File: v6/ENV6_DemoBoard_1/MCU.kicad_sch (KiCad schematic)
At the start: 41 parts, among them J401 Pico Debugger (SWD), J402 Conn_01x04_Pin, U401 RP2354B, U402 Pi-Radio, U403 W25Q16JVUXIQ, Y401 KX7_QRZ

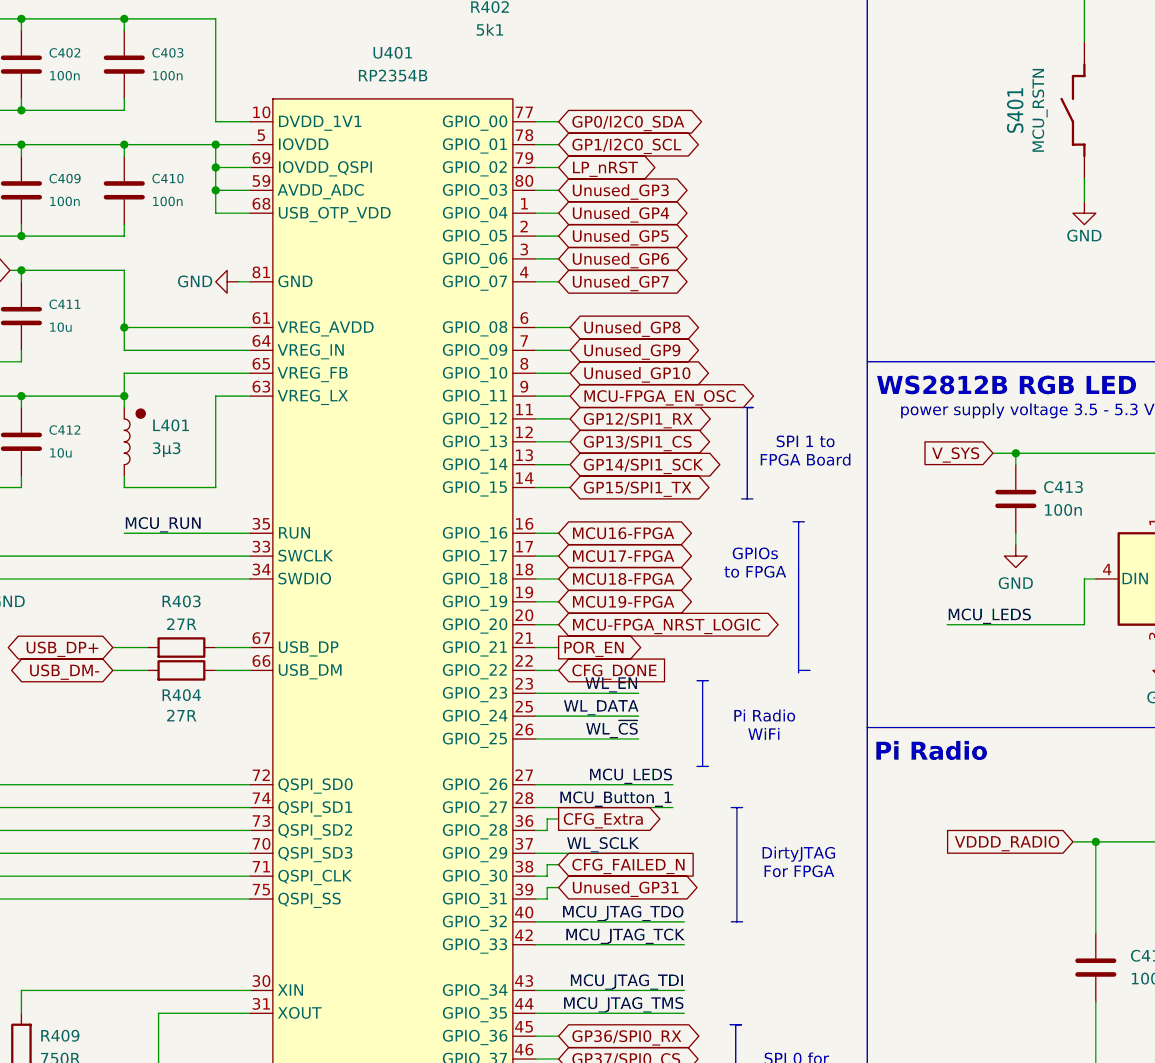
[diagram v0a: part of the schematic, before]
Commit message: first rev Base Board pcb layout
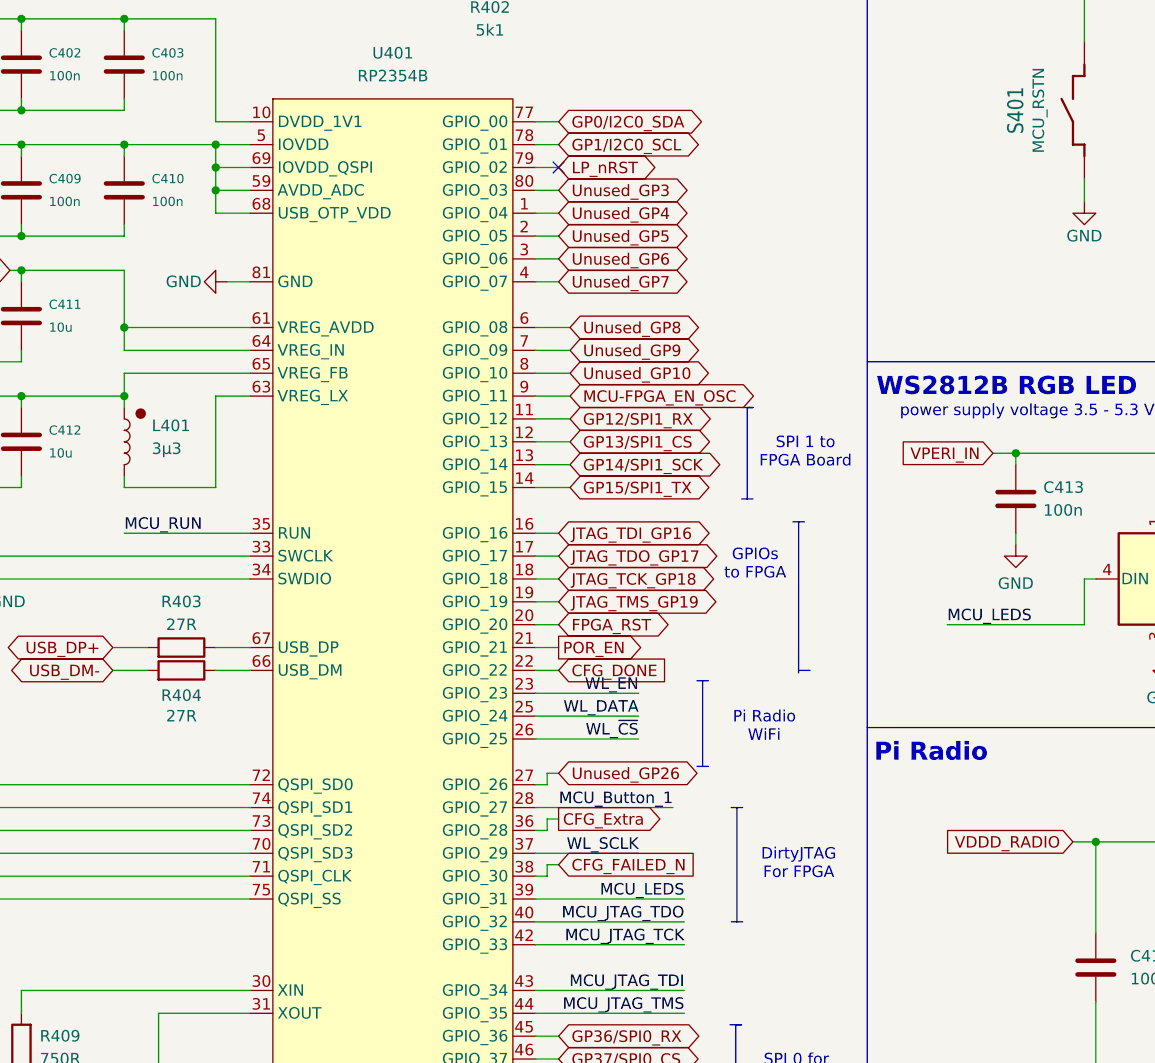
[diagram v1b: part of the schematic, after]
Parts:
- J401: footprint Connector_PinHeader_2.54mm:PinHeader_1x03_P2.54mm_Vertical -> Connector_PinHeader_2.00mm:PinHeader_1x03_P2.00mm_Vertical
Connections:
- net Unused_GP31 is gone; now on net MCU_LEDS: U401.39 (GPIO_31)
- net MCU_LEDS: no longer U401.27 (GPIO_26)
- net MCU-FPGA_NRST_LOGIC renamed FPGA_RST
- net MCU16-FPGA renamed JTAG_TDI_GP16
- net MCU17-FPGA renamed JTAG_TDO_GP17
- net MCU18-FPGA renamed JTAG_TCK_GP18
- net MCU19-FPGA renamed JTAG_TMS_GP19
- net V_SYS renamed VPERI_IN
- new net Unused_GP26: U401.27 (GPIO_26)
- no-connect marks 3 -> 4
